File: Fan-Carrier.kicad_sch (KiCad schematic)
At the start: 21 parts, among them J1 TC2030, J2 RJHSE-5381, M1 Fan_4pin, U1 AZ1117-3.3, U2 LM75

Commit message: added IDAnything
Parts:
- C1: IDAnything (none) -> 8ed1d4gh3rhtcap5n3thrqzk0z
- C2: IDAnything (none) -> 5es6p5fr8rkjdahcs3x36hwzw2
- C3: IDAnything (none) -> cjbd17kqpcg079c1ae8a37wt8d
- C4: IDAnything (none) -> 7306hr3vk0hr983c9yxsesf49q
- J2: IDAnything (none) -> ak2rtrj5wwjn58jx1er1822wfh
- M1: IDAnything (none) -> 14hyke6qq4k53atdbe9b9c6sqr
- R1, R2: IDAnything (none) -> 8qy9kfpz4rjz68060b2d6hntm0
- R3: IDAnything (none) -> e4khx4jva8k0wb08y4n5nr9g3p
- R4, R5, R6: IDAnything (none) -> ct46g33j3jkr389e4bd4v5859v
- U1: IDAnything (none) -> 3ykdfnd5ejg2s80rn0p5q546ag
- U2: IDAnything (none) -> 1fcznxzgv2j8g96pwsa7fzt0ca
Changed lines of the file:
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@@
+			)
+		)
+		(property "IDAnything" "8ed1d4gh3rhtcap5n3thrqzk0z"
+			(at 25.4 132.08 0)
+			(effects
+				(font
+					(size 1.27 1.27)
+				)
+				(hide yes)
 			)
 		)
@@
 			)
 		)
+		(property "IDAnything" "7306hr3vk0hr983c9yxsesf49q"
+			(at 222.25 115.57 0)
+			(effects
+				(font
+					(size 1.27 1.27)
+				)
+				(hide yes)
+			)
+		)
 		(pin "1"
 		)
@@
 			)
 		)
+		(property "IDAnything" "5es6p5fr8rkjdahcs3x36hwzw2"
+			(at 62.23 132.08 0)
+			(effects
+				(font
+					(size 1.27 1.27)
+				)
+				(hide yes)
+			)
+		)
 		(pin "1"
 		)
@@
 		)
 		(property "MOUSER#" "791-WR08X2700FTL"
+			(at 33.02 91.44 0)
+			(effects
+				(font
+					(size 1.27 1.27)
+				)
+				(hide yes)
+			)
+		)
+		(property "IDAnything" "8qy9kfpz4rjz68060b2d6hntm0"
 			(at 33.02 91.44 0)
 			(effects
@@
 			)
 		)
+		(property "IDAnything" "e4khx4jva8k0wb08y4n5nr9g3p"
+			(at 93.98 151.13 90)
+			(effects
+				(font
+					(size 1.27 1.27)
+				)
+				(hide yes)
+			)
+		)
 		(pin "1"
 		)
@@
 			)
 		)
+		(property "IDAnything" "ct46g33j3jkr389e4bd4v5859v"
+			(at 238.76 59.69 0)
+			(effects
+				(font
+					(size 1.27 1.27)
+				)
+				(hide yes)
+			)
+		)
 		(pin "1"
 		)
@@
 			)
 		)
+		(property "IDAnything" "ct46g33j3jkr389e4bd4v5859v"
+			(at 250.19 115.57 0)
+			(effects
+				(font
+					(size 1.27 1.27)
+				)
+				(hide yes)
+			)
+		)
 		(pin "1"
 		)
@@
 			)
 		)
+		(property "IDAnything" "3ykdfnd5ejg2s80rn0p5q546ag"
+			(at 44.45 125.73 0)
+			(effects
+				(font
+					(size 1.27 1.27)
+				)
+				(hide yes)
+			)
+		)
 		(pin "1"
 		)
@@
 			)
 		)
+		(property "IDAnything" "14hyke6qq4k53atdbe9b9c6sqr"
+			(at 252.73 71.12 0)
+			(effects
+				(font
+					(size 1.27 1.27)
+				)
+				(hide yes)
+			)
+		)
 		(pin "4"
 		)
@@
 			)
 		)
+		(property "IDAnything" "8qy9kfpz4rjz68060b2d6hntm0"
+			(at 33.02 76.2 0)
+			(effects
+				(font
+					(size 1.27 1.27)
+				)
+				(hide yes)
+			)
+		)
 		(pin "1"
 		)
@@
 			)
 		)
+		(property "IDAnything" "cjbd17kqpcg079c1ae8a37wt8d"
+			(at 154.94 138.43 90)
+			(effects
+				(font
+					(size 1.27 1.27)
+				)
+				(hide yes)
+			)
+		)
 		(pin "1"
 		)
@@
 			)
 		)
+		(property "IDAnything" "ct46g33j3jkr389e4bd4v5859v"
+			(at 259.08 115.57 0)
+			(effects
+				(font
+					(size 1.27 1.27)
+				)
+				(hide yes)
+			)
+		)
 		(pin "1"
 		)
@@
 			)
 		)
+		(property "IDAnything" "1fcznxzgv2j8g96pwsa7fzt0ca"
+			(at 234.95 125.73 0)
+			(effects
+				(font
+					(size 1.27 1.27)
+				)
+				(hide yes)
+			)
+		)
 		(pin "8"
 		)
@@
 			(at 53.34 83.82 0)
 			(effects
+				(font
+					(size 1.27 1.27)
+				)
+				(hide yes)
+			)
+		)
+		(property "IDAnything" "ak2rtrj5wwjn58jx1er1822wfh"
+			(at 53.34 83.82 0)
+			(effects

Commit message: increased thermal relief updated holddown nut solder paste pattern
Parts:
- J3: footprint openPoENode:119A-80A00-R02 -> openPoeNode:119A-80A00-R02
- J4: footprint openPoENode:119A-NUT-80-R02 -> openPoeNode:119A-NUT-80-R02
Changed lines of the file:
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@@
 			)
 		)
-		(property "Footprint" "openPoENode:119A-80A00-R02"
+		(property "Footprint" "openPoeNode:119A-80A00-R02"
 			(at 142.24 81.28 0)
 			(effects
@@
 			)
 		)
-		(property "Footprint" "openPoENode:119A-NUT-80-R02"
+		(property "Footprint" "openPoeNode:119A-NUT-80-R02"
 			(at 158.75 125.73 0)
 			(effects

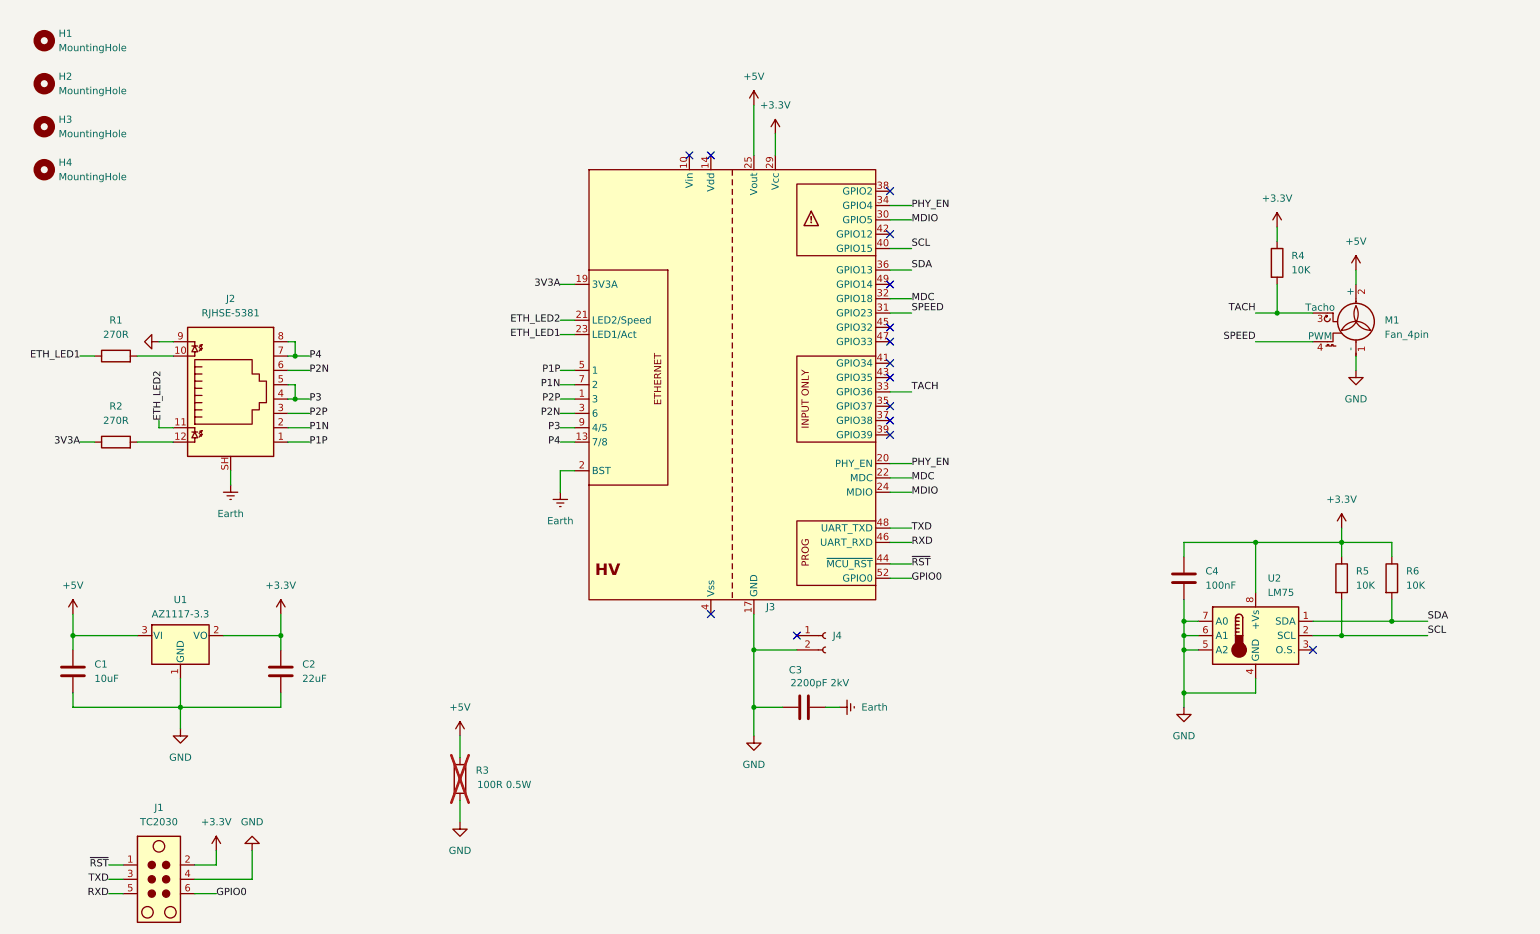
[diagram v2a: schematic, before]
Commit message: prettification
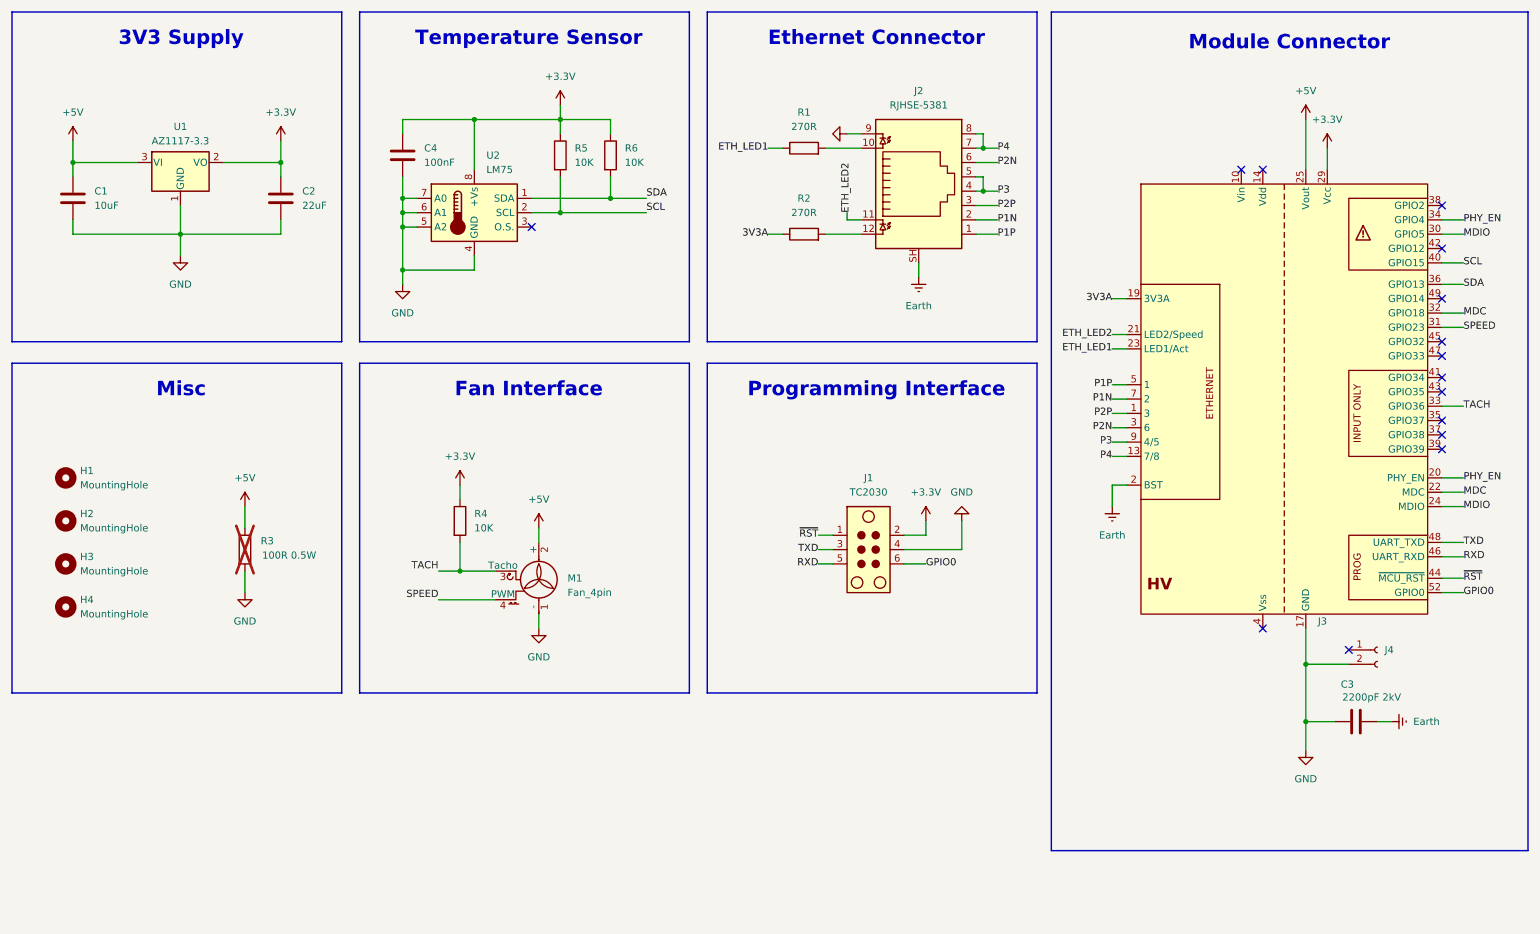
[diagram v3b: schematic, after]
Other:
- note added: "3V3 Supply"
- note added: "Ethernet Connector"
- note added: "Fan Interface"
- note added: "Misc"
- note added: "Module Connector"
- note added: "Programming Interface"
- note added: "Temperature Sensor"
- title: (none) -> openPoeNode Fan Carrier Board
- moved on the sheet: C1, C2, C3, C4, H1, H2, H3, H4, J1, J2, J3, J4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
